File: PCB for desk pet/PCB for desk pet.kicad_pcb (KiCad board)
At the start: 2 copper layers, 10 parts, among them J1 Conn_01x02, J2 Conn_01x04, J3 Conn_01x02, SW1 SW_SPDT, SW2 SW_Push, SW3 SW_Push

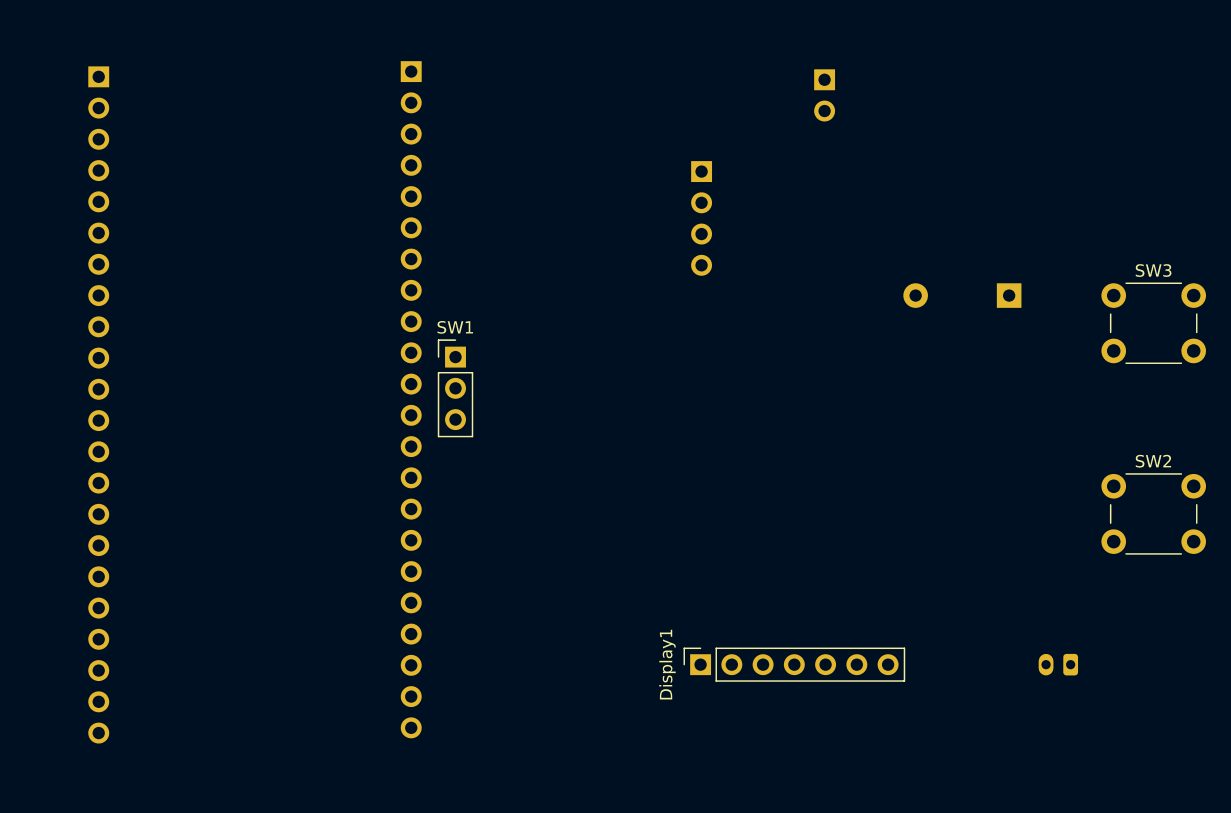
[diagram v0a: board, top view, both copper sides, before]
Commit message: PCB done
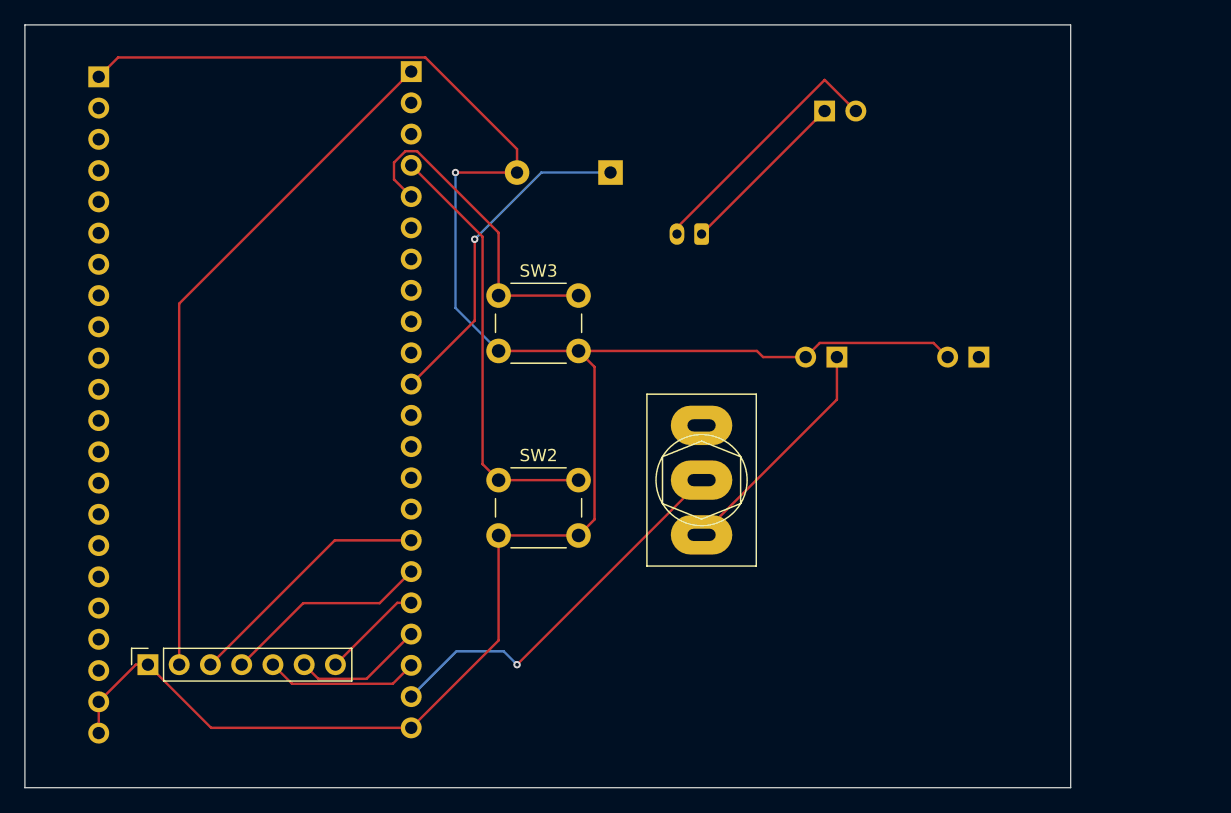
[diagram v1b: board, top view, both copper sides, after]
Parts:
- added J4: Conn_01x02, Connector_PinHeader_2.54mm:PinHeader_1x02_P2.54mm_Vertical, B.Cu at (176.0, 115.0)
- J2: value Conn_01x04 -> Conn_01x02; footprint Connector_PinHeader_2.54mm:PinHeader_1x04_P2.54mm_Vertical -> Connector_PinHeader_2.54mm:PinHeader_1x02_P2.54mm_Vertical
- SW1: footprint Connector_PinHeader_2.54mm:PinHeader_1x03_P2.54mm_Vertical -> extra:SW_Toggle_Blue_wSlots
- moved SW2 50.0 mm to (148.5, 125.0)
- moved SW3 50.0 mm to (148.5, 110.0)
- moved J3 46.1 mm to (165.0, 105.0)
- moved Display1 44.9 mm to (120.0, 140.0)
- moved BZ1 33.9 mm to (157.6, 100.0)
- moved J1 25.8 mm to (187.5, 115.0), turned to 90 degrees
- moved SW1 22.4 mm to (165.0, 125.0), turned to 90 degrees
- moved J2 11.1 mm to (175.0, 95.0), turned to -90 degrees
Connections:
- J2 pad 1: /V_UNSW -> /BAT+
- J2 pad 2: /VBAT -> /BAT-
- J3 pad 1: /VBAT -> /BAT+
- J3 pad 2: GND -> /BAT-
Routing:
- net GND: track 0.00 -> 170.7 mm, vias 0 -> 1
- net +3V3: track 0.00 -> 56.0 mm
- net /BTN_MENU: track 0.00 -> 35.0 mm
- net +5V: track 0.00 -> 31.8 mm, vias 0 -> 1
- net /BUZZER: track 0.00 -> 27.2 mm, vias 0 -> 1
- net /BTN_ACTION: track 0.00 -> 26.6 mm
- net /BAT-: track 0.00 -> 21.1 mm
- net /LCD_SCL: track 0.00 -> 20.5 mm
- net /V_UNSW: track 0.00 -> 19.0 mm
- net /LCD_SDA: track 0.00 -> 16.9 mm
- net /BAT+: track 0.00 -> 14.1 mm
- net /LCD_RES: track 0.00 -> 12.5 mm
- net /LCD_DC: track 0.00 -> 10.7 mm
- net /LCD_CS: track 0.00 -> 8.24 mm
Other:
- board outline added: 85 x 62 mm
